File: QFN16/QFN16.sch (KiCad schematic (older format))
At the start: 5 parts, among them J1 Conn_01x08, J2 Conn_02x08_Counter_Clockwise, J3 Conn_01x08, J4 Conn_02x08_Counter_Clockwise, J5 Conn_01x03

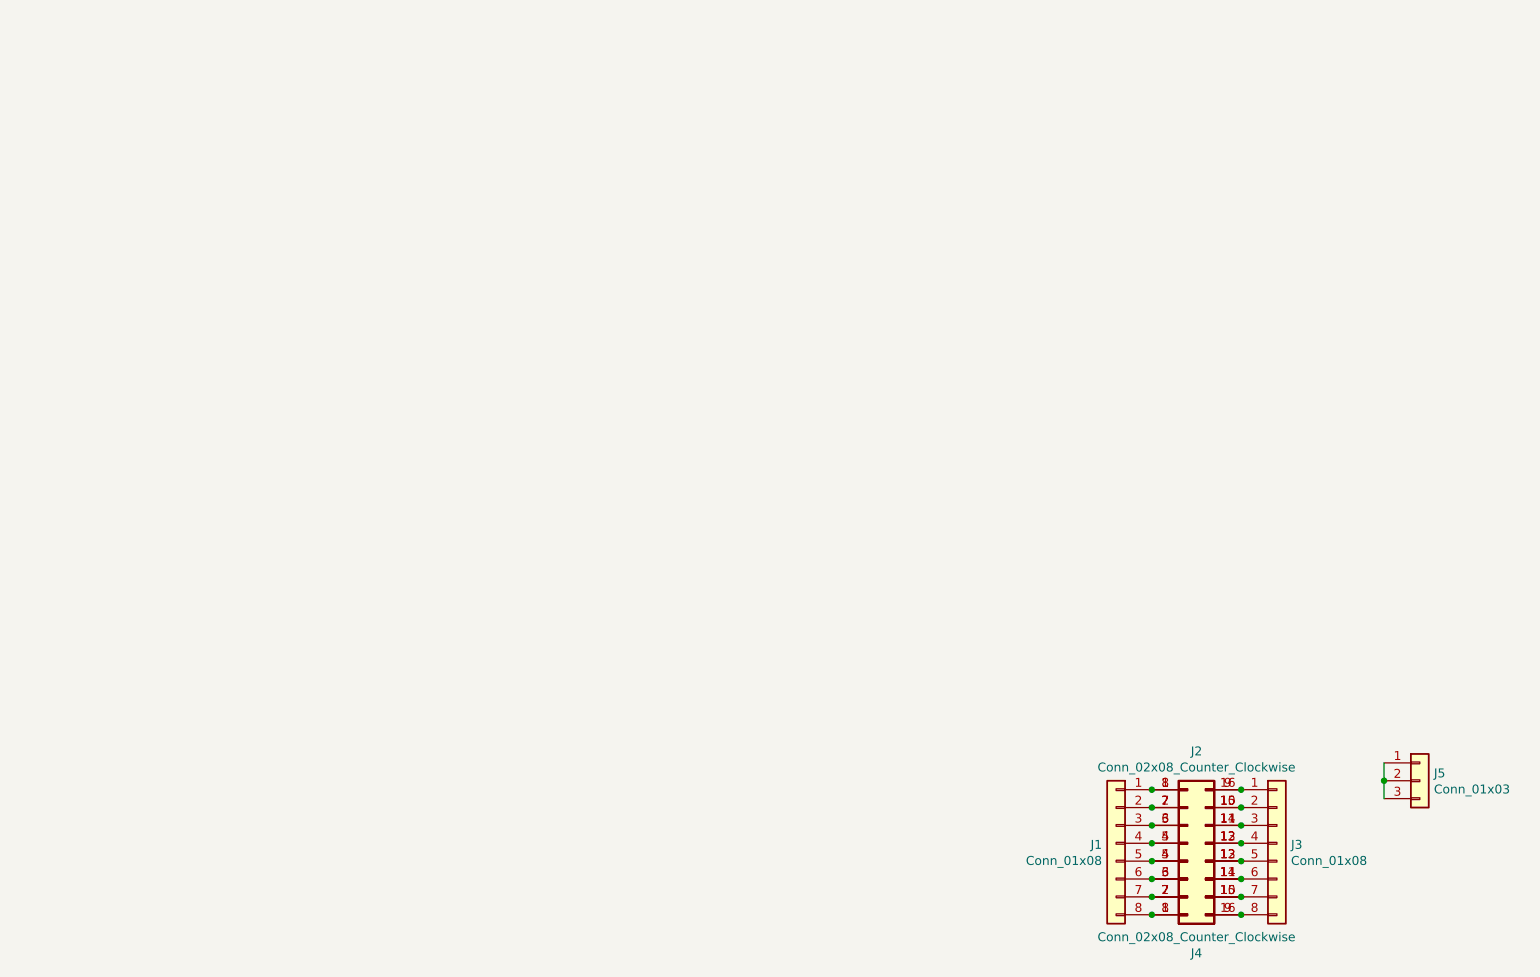
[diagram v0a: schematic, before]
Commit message: Page Settings Updated
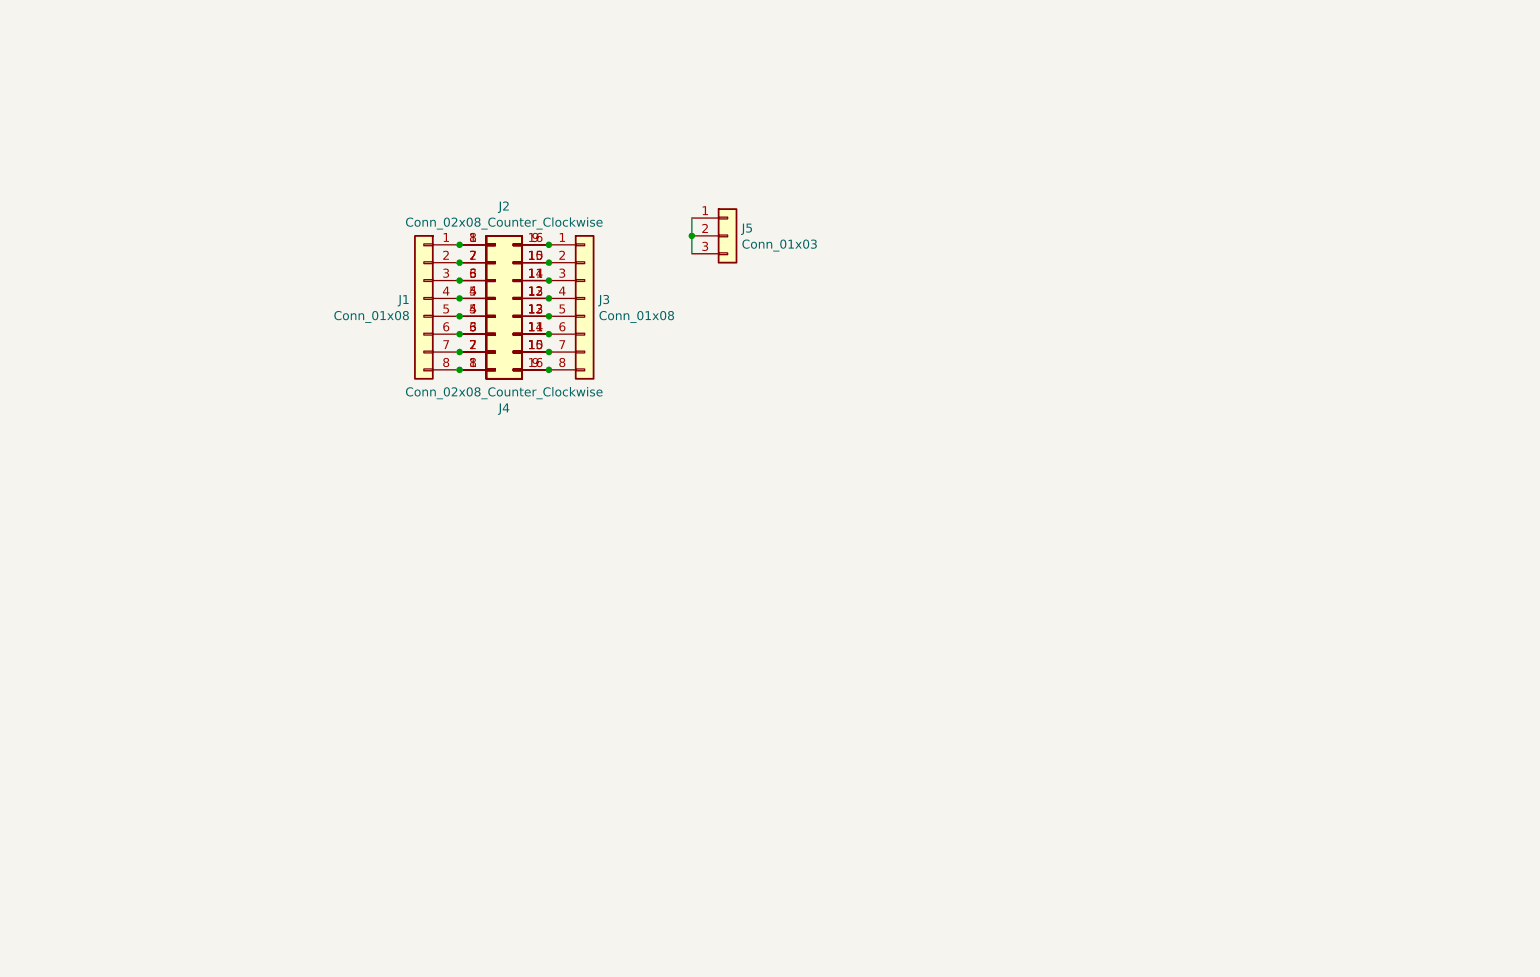
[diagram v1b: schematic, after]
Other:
- moved on the sheet: J1, J2, J3, J4, J5
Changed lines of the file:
@@
 EELAYER 29 0
 EELAYER END
-$Descr A4 11693 8268
+$Descr User 8268 5807
 encoding utf-8
 Sheet 1 1
@@
 L Connector_Generic:Conn_01x08 J3
 U 1 1 5D27708E
-P 8400 5500
-F 0 "J3" H 8479 5492 50  0000 L CNN
-F 1 "Conn_01x08" H 8479 5402 50  0000 L CNN
-F 2 "Connector_PinHeader_2.54mm:PinHeader_1x08_P2.54mm_Vertical" H 8400 5500 50  0001 C CNN
-F 3 "~" H 8400 5500 50  0001 C CNN
-	1    8400 5500
+P 4525 2450
+F 0 "J3" H 4604 2442 50  0000 L CNN
+F 1 "Conn_01x08" H 4604 2352 50  0000 L CNN
+F 2 "Connector_PinHeader_2.54mm:PinHeader_1x08_P2.54mm_Vertical" H 4525 2450 50  0001 C CNN
+F 3 "~" H 4525 2450 50  0001 C CNN
+	1    4525 2450
 	1    0    0    -1
 $EndComp
@@
 L Connector_Generic:Conn_02x08_Counter_Clockwise J2
 U 1 1 5D2772F5
-P 7900 5500
-F 0 "J2" H 7950 6015 50  0000 C CNN
-F 1 "Conn_02x08_Counter_Clockwise" H 7950 5925 50  0000 C CNN
-F 2 "Package_DFN_QFN:QFN-20-1EP_4x4mm_P0.5mm_EP2.7x2.7mm" H 7900 5500 50  0001 C CNN
-F 3 "~" H 7900 5500 50  0001 C CNN
-	1    7900 5500
+P 4025 2450
+F 0 "J2" H 4075 2965 50  0000 C CNN
+F 1 "Conn_02x08_Counter_Clockwise" H 4075 2875 50  0000 C CNN
+F 2 "Package_DFN_QFN:QFN-20-1EP_4x4mm_P0.5mm_EP2.7x2.7mm" H 4025 2450 50  0001 C CNN
+F 3 "~" H 4025 2450 50  0001 C CNN
+	1    4025 2450
 	1    0    0    -1
 $EndComp
@@
 L Connector_Generic:Conn_01x08 J1
 U 1 1 5D27904E
-P 7500 5500
-F 0 "J1" H 7579 5492 50  0000 L CNN
-F 1 "Conn_01x08" H 7579 5402 50  0000 L CNN
-F 2 "Connector_PinHeader_2.54mm:PinHeader_1x08_P2.54mm_Vertical" H 7500 5500 50  0001 C CNN
-F 3 "~" H 7500 5500 50  0001 C CNN
-	1    7500 5500
+P 3625 2450
+F 0 "J1" H 3704 2442 50  0000 L CNN
+F 1 "Conn_01x08" H 3704 2352 50  0000 L CNN
+F 2 "Connector_PinHeader_2.54mm:PinHeader_1x08_P2.54mm_Vertical" H 3625 2450 50  0001 C CNN
+F 3 "~" H 3625 2450 50  0001 C CNN
+	1    3625 2450
 	-1   0    0    -1
 $EndComp
@@
 L Connector_Generic:Conn_02x08_Counter_Clockwise J4
 U 1 1 5D27A0A0
-P 7900 5600
-F 0 "J4" H 7950 6115 50  0000 C CNN
-F 1 "Conn_02x08_Counter_Clockwise" H 7950 6025 50  0000 C CNN
-F 2 "Package_DFN_QFN:QFN-16-1EP_5x5mm_P0.8mm_EP2.7x2.7mm" H 7900 5600 50  0001 C CNN
-F 3 "~" H 7900 5600 50  0001 C CNN
-	1    7900 5600
+P 4025 2550
+F 0 "J4" H 4075 3065 50  0000 C CNN
+F 1 "Conn_02x08_Counter_Clockwise" H 4075 2975 50  0000 C CNN
+F 2 "Package_DFN_QFN:QFN-16-1EP_5x5mm_P0.8mm_EP2.7x2.7mm" H 4025 2550 50  0001 C CNN
+F 3 "~" H 4025 2550 50  0001 C CNN
+	1    4025 2550
 	1    0    0    1
 $EndComp
-Connection ~ 7700 5200
-Connection ~ 7700 5300
-Connection ~ 7700 5400
-Connection ~ 7700 5500
-Connection ~ 7700 5600
-Connection ~ 7700 5700
-Connection ~ 7700 5800
-Connection ~ 7700 5900
-Connection ~ 8200 5200
-Connection ~ 8200 5300
-Connection ~ 8200 5400
-Connection ~ 8200 5500
-Connection ~ 8200 5600
-Connection ~ 8200 5700
-Connection ~ 8200 5800
-Connection ~ 8200 5900
+Connection ~ 3825 2150
+Connection ~ 3825 2250
+Connection ~ 3825 2350
+Connection ~ 3825 2450
+Connection ~ 3825 2550
+Connection ~ 3825 2650
+Connection ~ 3825 2750
+Connection ~ 3825 2850
+Connection ~ 4325 2150
+Connection ~ 4325 2250
+Connection ~ 4325 2350
+Connection ~ 4325 2450
+Connection ~ 4325 2550
+Connection ~ 4325 2650
+Connection ~ 4325 2750
+Connection ~ 4325 2850
 $Comp
 L Connector_Generic:Conn_01x03 J5
 U 1 1 5D3B084D
-P 9200 5150
-F 0 "J5" H 9279 5192 50  0000 L CNN
-F 1 "Conn_01x03" H 9279 5102 50  0000 L CNN
-F 2 "Connector_PinHeader_2.54mm:PinHeader_1x03_P2.54mm_Vertical" H 9200 5150 50  0001 C CNN
-F 3 "~" H 9200 5150 50  0001 C CNN
-	1    9200 5150
+P 5325 2100
+F 0 "J5" H 5404 2142 50  0000 L CNN
+F 1 "Conn_01x03" H 5404 2052 50  0000 L CNN
+F 2 "Connector_PinHeader_2.54mm:PinHeader_1x03_P2.54mm_Vertical" H 5325 2100 50  0001 C CNN
+F 3 "~" H 5325 2100 50  0001 C CNN
+	1    5325 2100
 	1    0    0    -1
 $EndComp
 Wire Wire Line
-	9000 5050 9000 5150
-Connection ~ 9000 5150
+	5125 2000 5125 2100
+Connection ~ 5125 2100
 Wire Wire Line
-	9000 5150 9000 5250
+	5125 2100 5125 2200
 $EndSCHEMATC

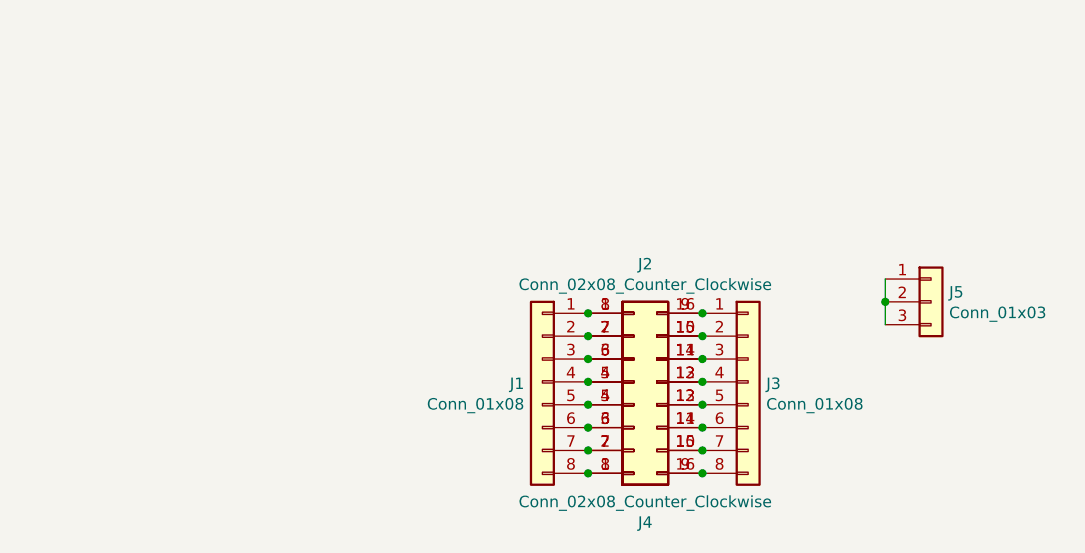
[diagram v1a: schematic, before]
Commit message: Schematic PDF and 3D Renders added
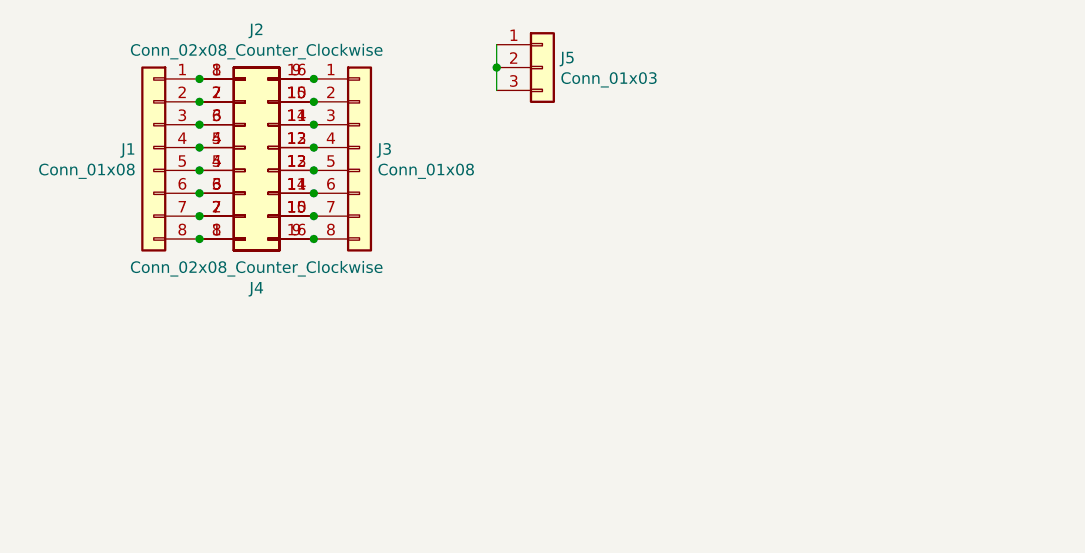
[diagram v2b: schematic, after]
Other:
- moved on the sheet: J1, J2, J3, J4, J5
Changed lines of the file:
@@
 EELAYER 29 0
 EELAYER END
-$Descr User 8268 5807
+$Descr User 5197 4016
 encoding utf-8
 Sheet 1 1
@@
 L Connector_Generic:Conn_01x08 J3
 U 1 1 5D27708E
-P 4525 2450
-F 0 "J3" H 4604 2442 50  0000 L CNN
-F 1 "Conn_01x08" H 4604 2352 50  0000 L CNN
-F 2 "Connector_PinHeader_2.54mm:PinHeader_1x08_P2.54mm_Vertical" H 4525 2450 50  0001 C CNN
-F 3 "~" H 4525 2450 50  0001 C CNN
-	1    4525 2450
+P 2825 1425
+F 0 "J3" H 2904 1417 50  0000 L CNN
+F 1 "Conn_01x08" H 2904 1327 50  0000 L CNN
+F 2 "Connector_PinHeader_2.54mm:PinHeader_1x08_P2.54mm_Vertical" H 2825 1425 50  0001 C CNN
+F 3 "~" H 2825 1425 50  0001 C CNN
+	1    2825 1425
 	1    0    0    -1
 $EndComp
@@
 L Connector_Generic:Conn_02x08_Counter_Clockwise J2
 U 1 1 5D2772F5
-P 4025 2450
-F 0 "J2" H 4075 2965 50  0000 C CNN
-F 1 "Conn_02x08_Counter_Clockwise" H 4075 2875 50  0000 C CNN
-F 2 "Package_DFN_QFN:QFN-20-1EP_4x4mm_P0.5mm_EP2.7x2.7mm" H 4025 2450 50  0001 C CNN
-F 3 "~" H 4025 2450 50  0001 C CNN
-	1    4025 2450
+P 2325 1425
+F 0 "J2" H 2375 1940 50  0000 C CNN
+F 1 "Conn_02x08_Counter_Clockwise" H 2375 1850 50  0000 C CNN
+F 2 "Package_DFN_QFN:QFN-20-1EP_4x4mm_P0.5mm_EP2.7x2.7mm" H 2325 1425 50  0001 C CNN
+F 3 "~" H 2325 1425 50  0001 C CNN
+	1    2325 1425
 	1    0    0    -1
 $EndComp
@@
 L Connector_Generic:Conn_01x08 J1
 U 1 1 5D27904E
-P 3625 2450
-F 0 "J1" H 3704 2442 50  0000 L CNN
-F 1 "Conn_01x08" H 3704 2352 50  0000 L CNN
-F 2 "Connector_PinHeader_2.54mm:PinHeader_1x08_P2.54mm_Vertical" H 3625 2450 50  0001 C CNN
-F 3 "~" H 3625 2450 50  0001 C CNN
-	1    3625 2450
+P 1925 1425
+F 0 "J1" H 2004 1417 50  0000 L CNN
+F 1 "Conn_01x08" H 2004 1327 50  0000 L CNN
+F 2 "Connector_PinHeader_2.54mm:PinHeader_1x08_P2.54mm_Vertical" H 1925 1425 50  0001 C CNN
+F 3 "~" H 1925 1425 50  0001 C CNN
+	1    1925 1425
 	-1   0    0    -1
 $EndComp
@@
 L Connector_Generic:Conn_02x08_Counter_Clockwise J4
 U 1 1 5D27A0A0
-P 4025 2550
-F 0 "J4" H 4075 3065 50  0000 C CNN
-F 1 "Conn_02x08_Counter_Clockwise" H 4075 2975 50  0000 C CNN
-F 2 "Package_DFN_QFN:QFN-16-1EP_5x5mm_P0.8mm_EP2.7x2.7mm" H 4025 2550 50  0001 C CNN
-F 3 "~" H 4025 2550 50  0001 C CNN
-	1    4025 2550
+P 2325 1525
+F 0 "J4" H 2375 2040 50  0000 C CNN
+F 1 "Conn_02x08_Counter_Clockwise" H 2375 1950 50  0000 C CNN
+F 2 "Package_DFN_QFN:QFN-16-1EP_5x5mm_P0.8mm_EP2.7x2.7mm" H 2325 1525 50  0001 C CNN
+F 3 "~" H 2325 1525 50  0001 C CNN
+	1    2325 1525
 	1    0    0    1
 $EndComp
-Connection ~ 3825 2150
-Connection ~ 3825 2250
-Connection ~ 3825 2350
-Connection ~ 3825 2450
-Connection ~ 3825 2550
-Connection ~ 3825 2650
-Connection ~ 3825 2750
-Connection ~ 3825 2850
-Connection ~ 4325 2150
-Connection ~ 4325 2250
-Connection ~ 4325 2350
-Connection ~ 4325 2450
-Connection ~ 4325 2550
-Connection ~ 4325 2650
-Connection ~ 4325 2750
-Connection ~ 4325 2850
+Connection ~ 2125 1125
+Connection ~ 2125 1225
+Connection ~ 2125 1325
+Connection ~ 2125 1425
+Connection ~ 2125 1525
+Connection ~ 2125 1625
+Connection ~ 2125 1725
+Connection ~ 2125 1825
+Connection ~ 2625 1125
+Connection ~ 2625 1225
+Connection ~ 2625 1325
+Connection ~ 2625 1425
+Connection ~ 2625 1525
+Connection ~ 2625 1625
+Connection ~ 2625 1725
+Connection ~ 2625 1825
 $Comp
 L Connector_Generic:Conn_01x03 J5
 U 1 1 5D3B084D
-P 5325 2100
-F 0 "J5" H 5404 2142 50  0000 L CNN
-F 1 "Conn_01x03" H 5404 2052 50  0000 L CNN
-F 2 "Connector_PinHeader_2.54mm:PinHeader_1x03_P2.54mm_Vertical" H 5325 2100 50  0001 C CNN
-F 3 "~" H 5325 2100 50  0001 C CNN
-	1    5325 2100
+P 3625 1075
+F 0 "J5" H 3704 1117 50  0000 L CNN
+F 1 "Conn_01x03" H 3704 1027 50  0000 L CNN
+F 2 "Connector_PinHeader_2.54mm:PinHeader_1x03_P2.54mm_Vertical" H 3625 1075 50  0001 C CNN
+F 3 "~" H 3625 1075 50  0001 C CNN
+	1    3625 1075
 	1    0    0    -1
 $EndComp
 Wire Wire Line
-	5125 2000 5125 2100
-Connection ~ 5125 2100
+	3425 975  3425 1075
+Connection ~ 3425 1075
 Wire Wire Line
-	5125 2100 5125 2200
+	3425 1075 3425 1175
 $EndSCHEMATC
